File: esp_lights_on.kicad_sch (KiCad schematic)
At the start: 0 parts

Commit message: some commits
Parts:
- added C1: 10uF, Capacitor_SMD:C_1210_3225Metric_Pad1.33x2.70mm_HandSolder, symbol Device:C
- added C2: 10uF, Capacitor_SMD:C_0805_2012Metric_Pad1.18x1.45mm_HandSolder, symbol Device:C
- added C3, C4: 100nF, Capacitor_SMD:C_0805_2012Metric_Pad1.18x1.45mm_HandSolder, symbol Device:C
- added D1: D, Diode_SMD:D_SMA_Handsoldering, symbol Device:D
- added J1: Conn_01x04_Pin, Connector_PinHeader_2.54mm:PinHeader_1x04_P2.54mm_Vertical, symbol Connector:Conn_01x04_Pin
- added J2: VOUT, TerminalBlock_Phoenix:TerminalBlock_Phoenix_MKDS-1,5-2-5.08_1x02_P5.08mm_Horizontal, symbol Connector:Screw_Terminal_01x02
- added J3: VIN, TerminalBlock_Phoenix:TerminalBlock_Phoenix_MKDS-1,5-2-5.08_1x02_P5.08mm_Horizontal, symbol Connector:Screw_Terminal_01x02
- added K1: RELAY, Relay_THT:Relay_SPST_Panasonic_ADW11, symbol Relay:ADW11
- added PS1: POWER, RACM06E-12SK_277:CONV_RACM06E-12SK_277, symbol RACM06E-12SK_277:RACM06E-12SK_277
- added Q1: SS8050, Package_TO_SOT_SMD:SOT-23-3, symbol Transistor_BJT:SS8050
- added R1: 1k, Resistor_SMD:R_1206_3216Metric_Pad1.30x1.75mm_HandSolder, symbol Device:R
- added U1: ESP32-WROOM-32, RF_Module:ESP32-WROOM-32, symbol RF_Module:ESP32-WROOM-32
- added U2: TLV1117-33, Package_TO_SOT_SMD:SOT-223-3_TabPin2, symbol Regulator_Linear:TLV1117-33
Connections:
- new net: Q1.1 (B), R1.2
- new net: C2.2, C3.2
- new net +3.3V: C2.1, C3.1, C4.1, U1.2 (VDD), U2.2 (VO)
- new net COLECTOR: D1.2 (A), K1.A2, Q1.3 (C)
- new net GND: C1.2, C4.2, J1.4 (Pin_4), PS1.4 (-VOUT), Q1.2 (E), U1.1 (GND), U1.15 (GND), U1.38 (GND), U1.39 (GND), U2.1 (GND)
- new net RX: J1.2 (Pin_2), U1.35 (TXD0/IO1)
- new net SW: R1.1, U1.33 (IO21)
- new net TX: J1.3 (Pin_3), U1.34 (RXD0/IO3)
- new net VIN_220V: J3.1 (Pin_1), K1.13, PS1.1 (VAC_IN(L))
- new net VIN_NULL: J2.1 (Pin_1), J3.2 (Pin_2), PS1.2 (VAC_IN(N))
- new net VOUT_220V: J2.2 (Pin_2), K1.14
- new net VOUT_5V: C1.1, D1.1 (K), J1.1 (Pin_1), K1.A1, PS1.5 (+VOUT), U2.3 (VI)

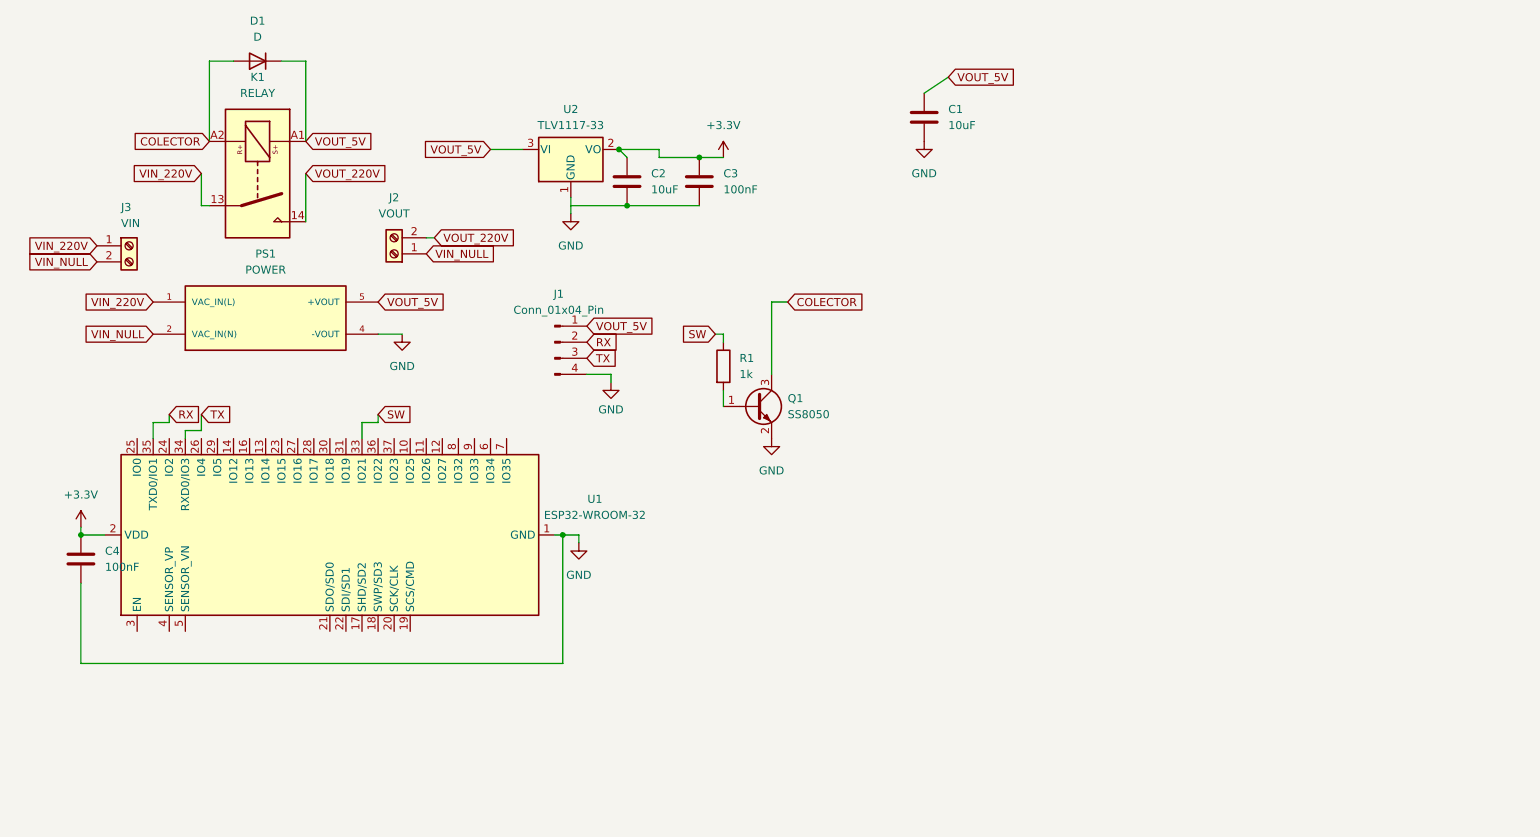
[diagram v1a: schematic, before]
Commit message: modification by ovi
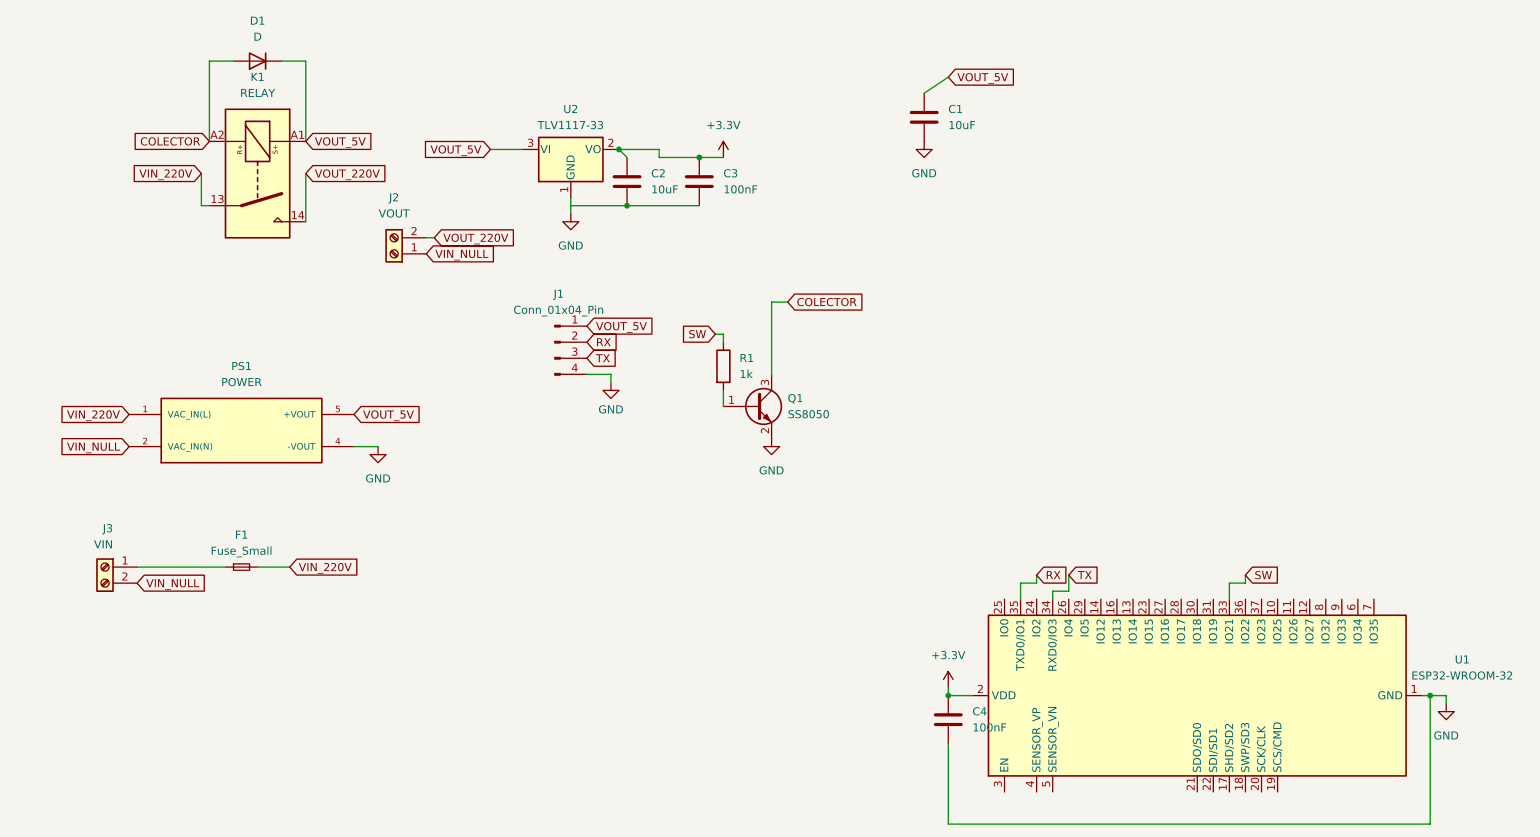
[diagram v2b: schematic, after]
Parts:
- added F1: Fuse_Small, Fuse:Fuse_Schurter_UMZ250, symbol Device:Fuse_Small
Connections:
- net VIN_220V: now also F1.2; no longer J3.1 (Pin_1)
- new net: F1.1, J3.1 (Pin_1)
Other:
- moved on the sheet: C4, J3, PS1, U1
